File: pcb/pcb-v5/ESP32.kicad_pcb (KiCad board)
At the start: 2 copper layers, 49 x 49 mm, 1 part

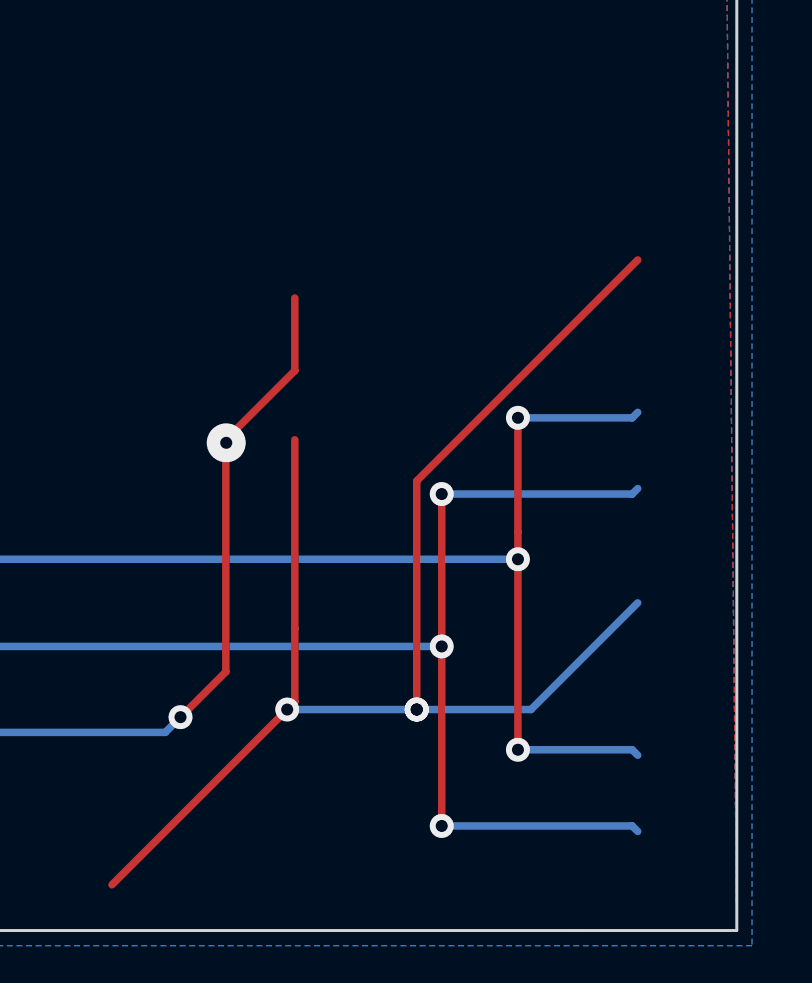
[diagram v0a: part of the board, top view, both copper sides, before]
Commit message: PCB-V5 update
PCB updated for presentation
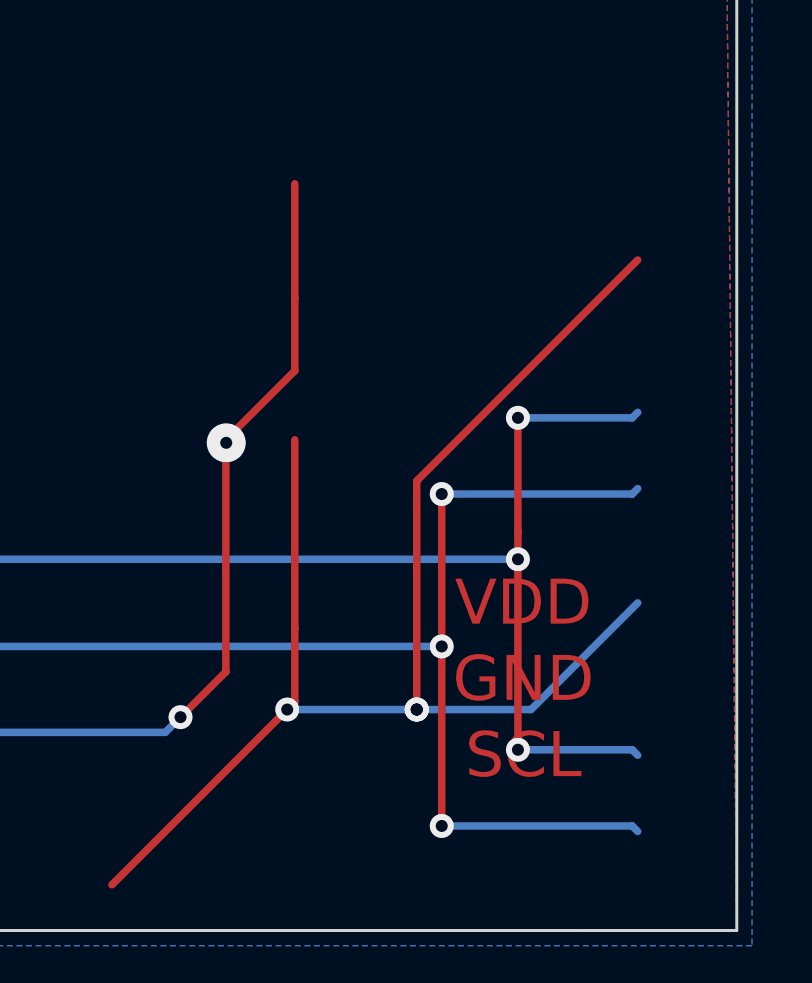
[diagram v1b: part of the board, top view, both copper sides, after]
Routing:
- net VIN: track 44.2 -> 48.0 mm
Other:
- board text added: "GND"
- board text added: "SCL"
- board text added: "SDA"
- board text added: "VDD"
